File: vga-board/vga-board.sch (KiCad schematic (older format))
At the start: 24 parts, among them J1 EXP, J2 EXP, J3 Conn_02x05_Odd_Even, U1 XC95144XL-TQ100, U2 IS61C5128AL-10TLI, X1 50MHz

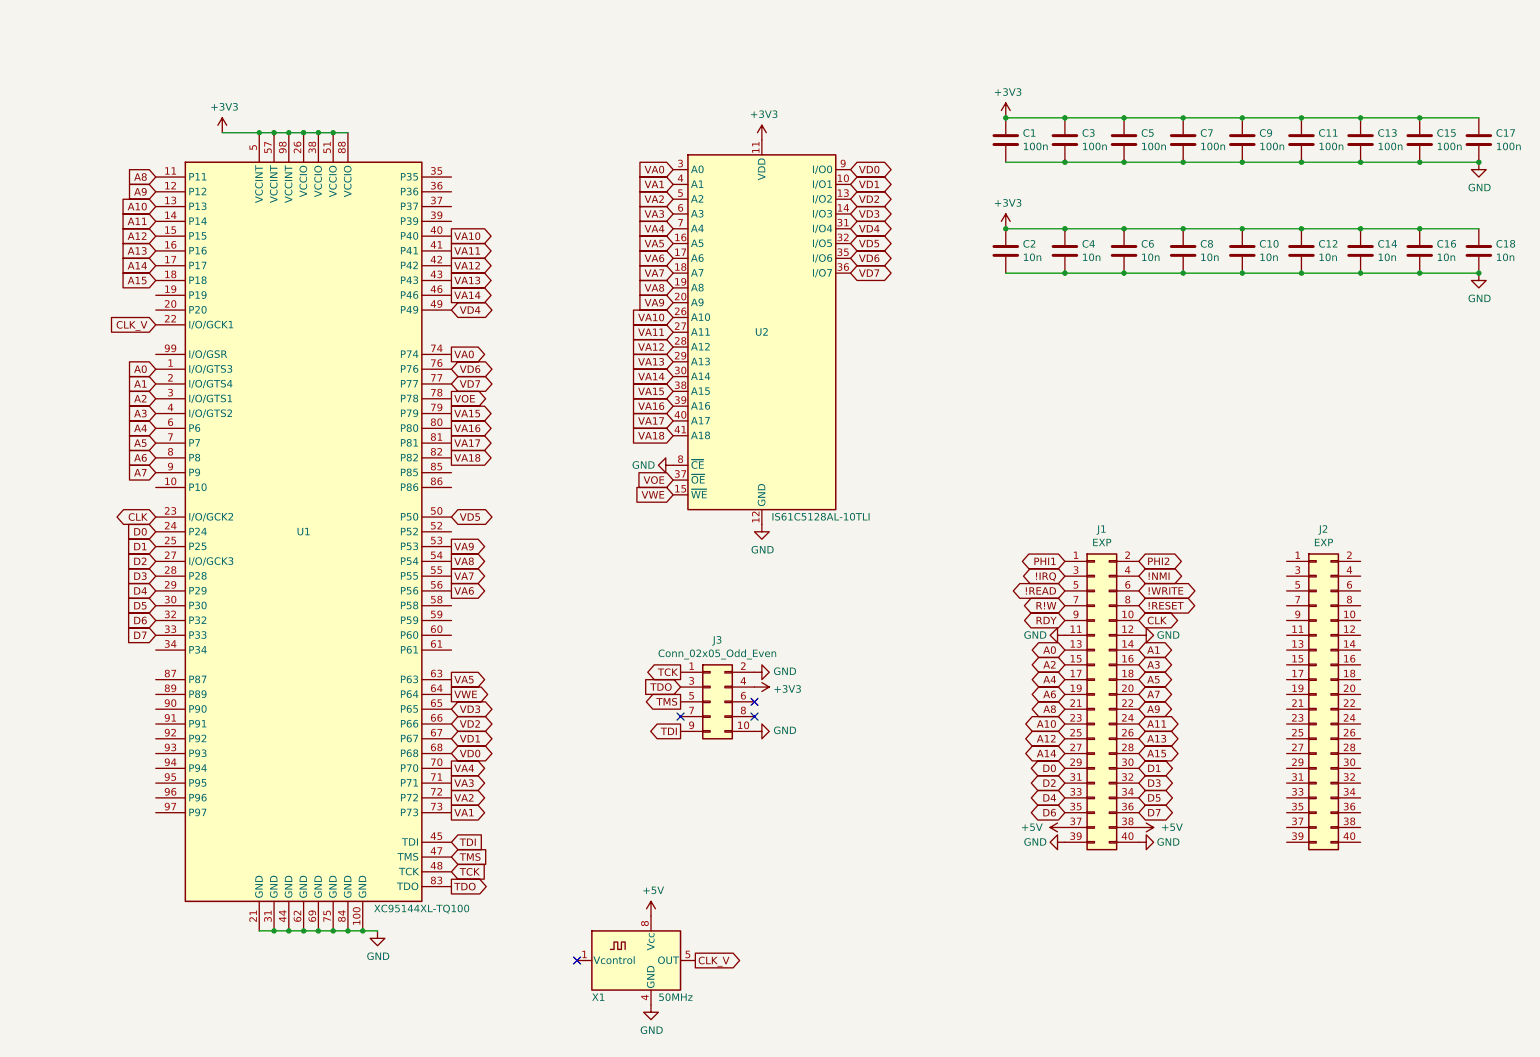
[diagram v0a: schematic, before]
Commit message: more vga board routing
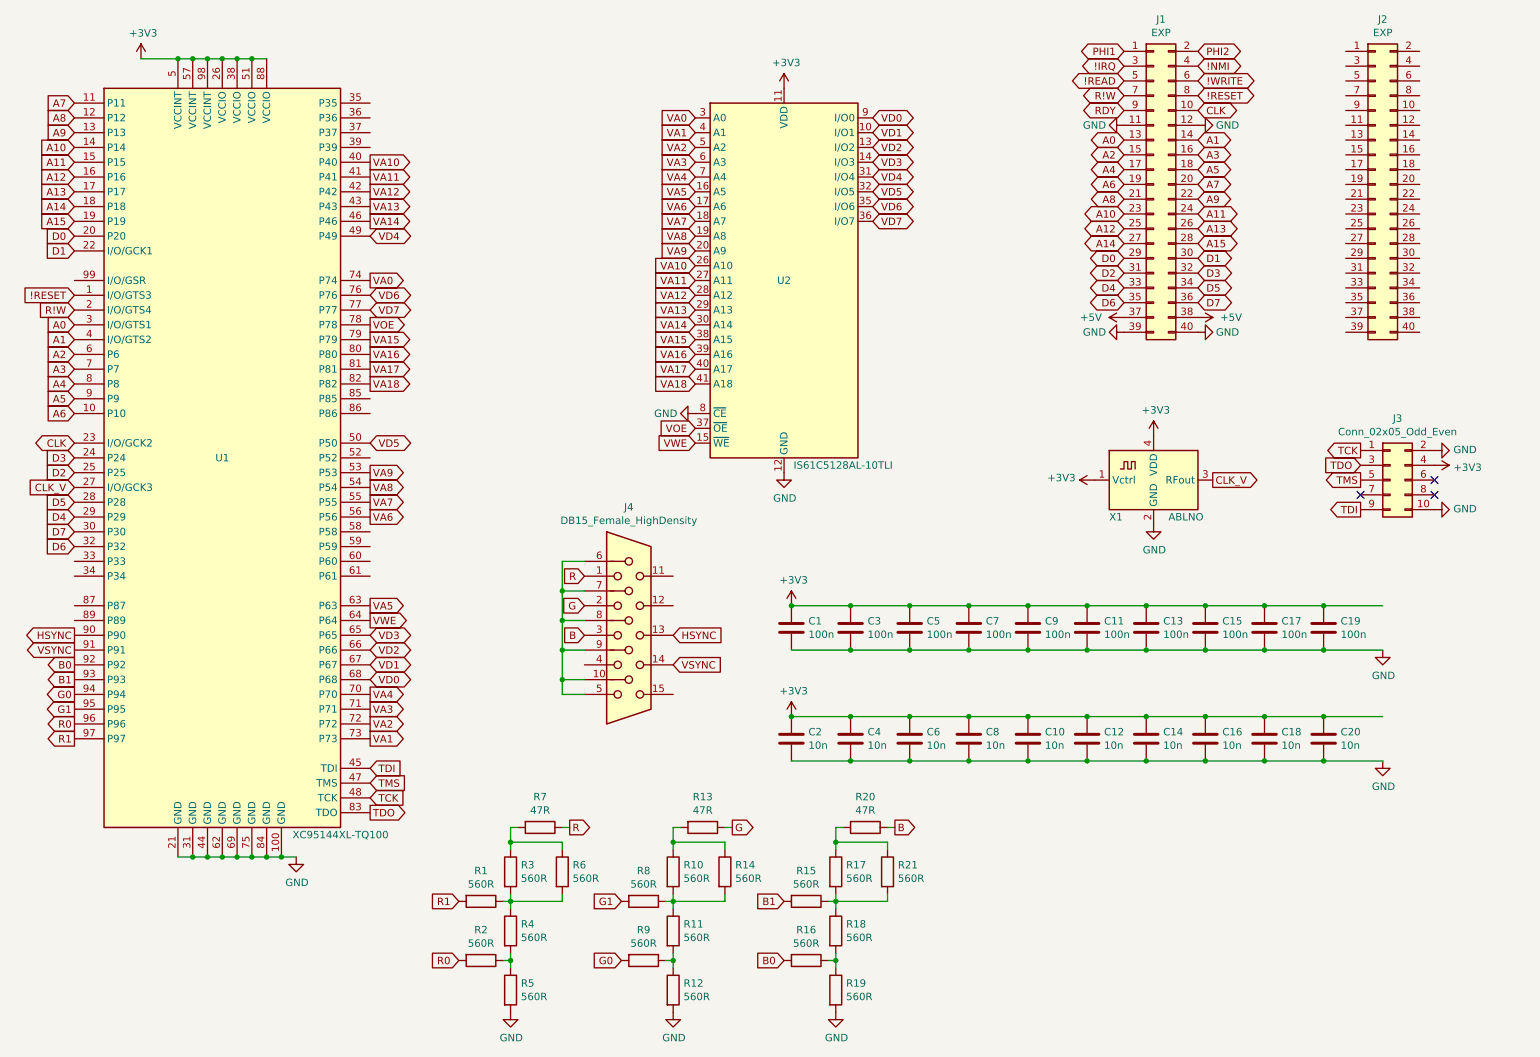
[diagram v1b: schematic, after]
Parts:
- removed X1: 50MHz, Oscillator:Oscillator_DIP-8, symbol Oscillator:VC-83
- added C19: 100n, Capacitor_SMD:C_0402_1005Metric, symbol Device:C
- added C20: 10n, Capacitor_SMD:C_0402_1005Metric, symbol Device:C
- added J4: DB15_Female_HighDensity, Connector_Dsub:DSUB-15-HD_Female_Horizontal_P2.29x1.98mm_EdgePinOffset3.03mm_Housed_MountingHolesOffset4.94mm, symbol Connector:DB15_Female_HighDensity
- added R1, R10, R11, R12, R14, R15, R16, R17, R18, R19, R2, R21, R3, R4, R5, R6, R8, R9: 560R, Resistor_SMD:R_0402_1005Metric, symbol Device:R
- added R13, R20, R7: 47R, Resistor_SMD:R_0402_1005Metric, symbol Device:R
- added X1: ABLNO, Oscillator:Oscillator_SMD_Abracon_ASV-4Pin_7.0x5.1mm, symbol Oscillator:ABLNO
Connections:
- net !RESET: now also U1.1 (I/O/GTS3)
- net +3V3: now also C19.1, C20.1, X1.1 (Vctrl), X1.4 (VDD)
- net A0: now also U1.3 (I/O/GTS1); no longer U1.1 (I/O/GTS3)
- net A1: now also U1.4 (I/O/GTS2); no longer U1.2 (I/O/GTS4)
- net A10: now also U1.14 (P14); no longer U1.13 (P13)
- net A11: now also U1.15 (P15); no longer U1.14 (P14)
- net A12: now also U1.16 (P16); no longer U1.15 (P15)
- net A13: now also U1.17 (P17); no longer U1.16 (P16)
- net A14: now also U1.18 (P18); no longer U1.17 (P17)
- net A15: now also U1.19 (P19); no longer U1.18 (P18)
- net A2: now also U1.6 (P6); no longer U1.3 (I/O/GTS1)
- net A3: now also U1.7 (P7); no longer U1.4 (I/O/GTS2)
- net A4: now also U1.8 (P8); no longer U1.6 (P6)
- net A5: now also U1.9 (P9); no longer U1.7 (P7)
- net A6: now also U1.10 (P10); no longer U1.8 (P8)
- net A7: now also U1.11 (P11); no longer U1.9 (P9)
- net A8: now also U1.12 (P12); no longer U1.11 (P11)
- net A9: now also U1.13 (P13); no longer U1.12 (P12)
- net CLK_V: now also U1.27 (I/O/GCK3), X1.3 (RFout); no longer U1.22 (I/O/GCK1)
- net D0: now also U1.20 (P20); no longer U1.24 (P24)
- net D1: now also U1.22 (I/O/GCK1); no longer U1.25 (P25)
- net D2: now also U1.25 (P25); no longer U1.27 (I/O/GCK3)
- net D3: now also U1.24 (P24); no longer U1.28 (P28)
- net D5: now also U1.28 (P28); no longer U1.30 (P30)
- net D7: now also U1.30 (P30); no longer U1.33 (P33)
- net GND: now also C19.2, C20.2, R12.2, R19.2, R5.2, X1.2 (GND)
- net R!W: now also U1.2 (I/O/GTS4)
- net HSYNC: now reaches U1.90 (P90)
- net HSYNC: now also J4.13
- net VSYNC: now reaches U1.91 (P91)
- net VSYNC: now also J4.14
- net B0: now reaches U1.92 (P92)
- net B0: now also R16.2
- net B1: now reaches U1.93 (P93)
- net B1: now also R15.2
- net G0: now reaches U1.94 (P94)
- net G0: now also R9.2
- net G1: now reaches U1.95 (P95)
- net G1: now also R8.2
- net R0: now reaches U1.96 (P96)
- net R0: now also R2.2
- net R1: now reaches U1.97 (P97)
- net R1: now also R1.2
- new net: R1.1, R3.2, R4.1, R6.2
- new net: R2.1, R4.2, R5.1
- new net: R3.1, R6.1, R7.2
- new net: R10.2, R11.1, R14.2, R8.1
- new net: R11.2, R12.1, R9.1
- new net: R10.1, R13.2, R14.1
- new net: R15.1, R17.2, R18.1, R21.2
- new net: R16.1, R18.2, R19.1
- new net: R17.1, R20.2, R21.1
- new net: J4.10, J4.5, J4.6, J4.7, J4.8, J4.9
- new net B: J4.3, R20.1
- new net G: J4.2, R13.1
- new net R: J4.1, R7.1
- no-connect marks 4 -> 3
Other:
- moved on the sheet: C1, C10, C11, C12, C13, C14, C15, C16, C2, C3, C4, C5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
